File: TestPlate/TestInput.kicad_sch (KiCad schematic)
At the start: 8 parts, among them U1 CD74HC4094E, U2 CD74HC4094E, U3 CD74HC4094E, U4 CD74HC4094E

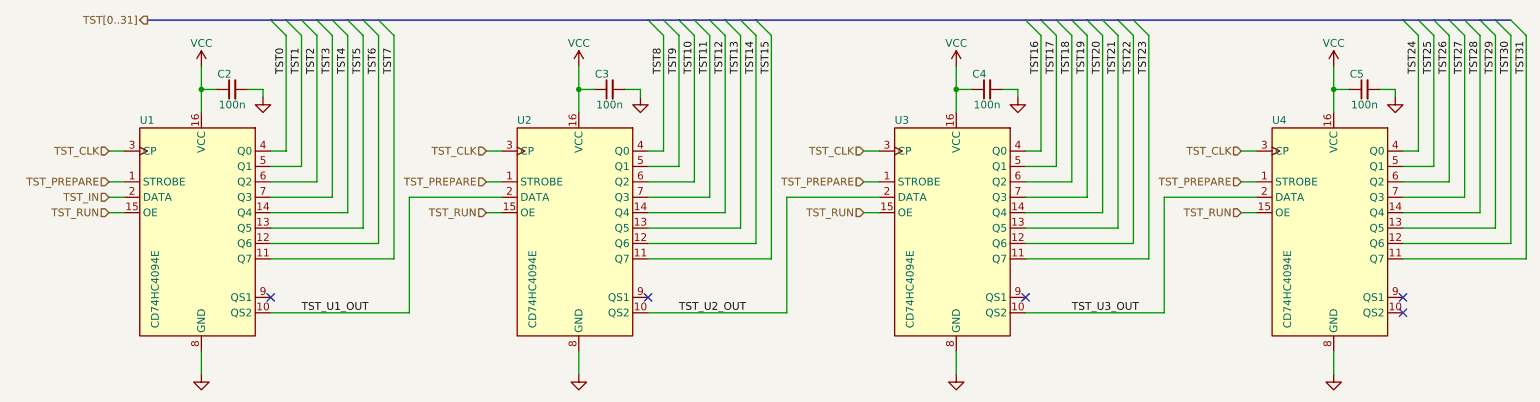
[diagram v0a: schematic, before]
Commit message: Some directory cleanup and structuring.
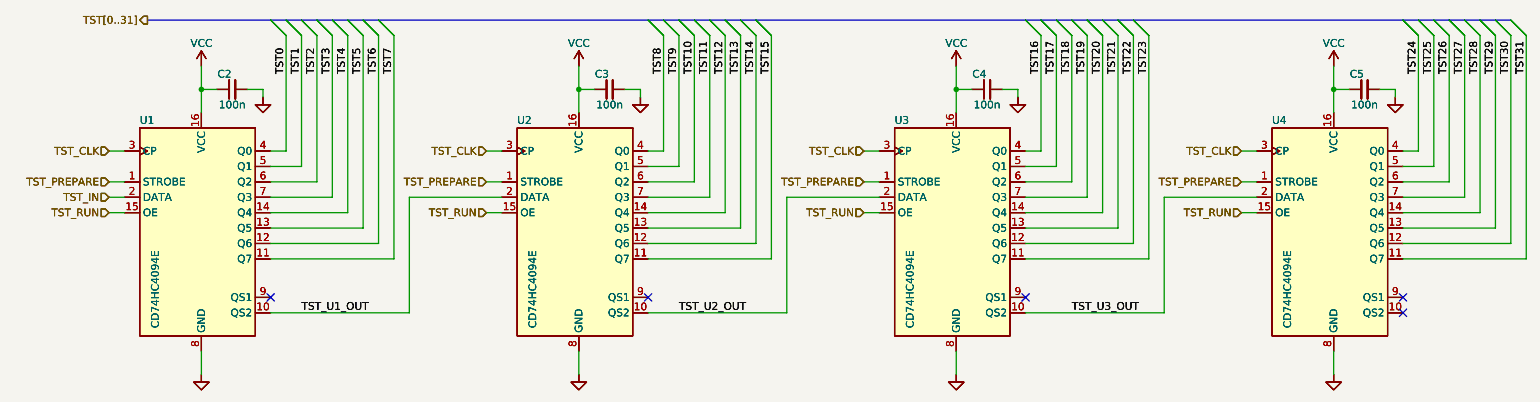
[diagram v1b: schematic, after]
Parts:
- added C2, C3, C4, C5: 100n, Capacitor_SMD:C_1206_3216Metric_Pad1.33x1.80mm_HandSolder, symbol Device:C_Small
- added U1, U2, U3, U4: CD74HC4094E, Package_DIP:DIP-16_W7.62mm_Socket, symbol CustomParts:CD74HC4094E
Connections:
- net GND: now also C2.2, C3.2, C4.2, C5.2, U1.8 (GND), U2.8 (GND), U3.8 (GND), U4.8 (GND)
- net TST0: now also U1.4 (Q0)
- net TST1: now also U1.5 (Q1)
- net TST10: now also U2.6 (Q2)
- net TST11: now also U2.7 (Q3)
- net TST12: now also U2.14 (Q4)
- net TST13: now also U2.13 (Q5)
- net TST14: now also U2.12 (Q6)
- net TST15: now also U2.11 (Q7)
- net TST16: now also U3.4 (Q0)
- net TST17: now also U3.5 (Q1)
- net TST18: now also U3.6 (Q2)
- net TST19: now also U3.7 (Q3)
- net TST2: now also U1.6 (Q2)
- net TST20: now also U3.14 (Q4)
- net TST21: now also U3.13 (Q5)
- net TST22: now also U3.12 (Q6)
- net TST23: now also U3.11 (Q7)
- net TST24: now also U4.4 (Q0)
- net TST25: now also U4.5 (Q1)
- net TST26: now also U4.6 (Q2)
- net TST27: now also U4.7 (Q3)
- net TST28: now also U4.14 (Q4)
- net TST29: now also U4.13 (Q5)
- net TST3: now also U1.7 (Q3)
- net TST30: now also U4.12 (Q6)
- net TST31: now also U4.11 (Q7)
- net TST4: now also U1.14 (Q4)
- net TST5: now also U1.13 (Q5)
- net TST6: now also U1.12 (Q6)
- net TST7: now also U1.11 (Q7)
- net TST8: now also U2.4 (Q0)
- net TST9: now also U2.5 (Q1)
- net TST_CLK: now also U1.3 (CP), U2.3 (CP), U3.3 (CP), U4.3 (CP)
- net TST_IN: now also U1.2 (DATA)
- net TST_PREPARE: now also U1.1 (STROBE), U2.1 (STROBE), U3.1 (STROBE), U4.1 (STROBE)
- net TST_RUN: now also U1.15 (OE), U2.15 (OE), U3.15 (OE), U4.15 (OE)
- net TST_U1_OUT: now also U1.10 (QS2), U2.2 (DATA)
- net TST_U2_OUT: now also U2.10 (QS2), U3.2 (DATA)
- net TST_U3_OUT: now also U3.10 (QS2), U4.2 (DATA)
- net VCC: now also C2.1, C3.1, C4.1, C5.1, U1.16 (VCC), U2.16 (VCC), U3.16 (VCC), U4.16 (VCC)
- net at U4.10 (QS2): now also U4.10 (QS2)
- net at U4.9 (QS1): now also U4.9 (QS1)
- net at U3.9 (QS1): now also U3.9 (QS1)
- net at U2.9 (QS1): now also U2.9 (QS1)
- net at U1.9 (QS1): now also U1.9 (QS1)
